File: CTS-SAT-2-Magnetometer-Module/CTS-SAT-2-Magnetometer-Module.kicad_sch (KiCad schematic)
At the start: 32 parts, among them J1 Conn_01x04_Pin, J2 SWD, SW1 SW_Push, U1 MMC5983MA, U2 LIS2MDL, U3 STM32F072C8Tx, U5 MIC5365-3.0YC5

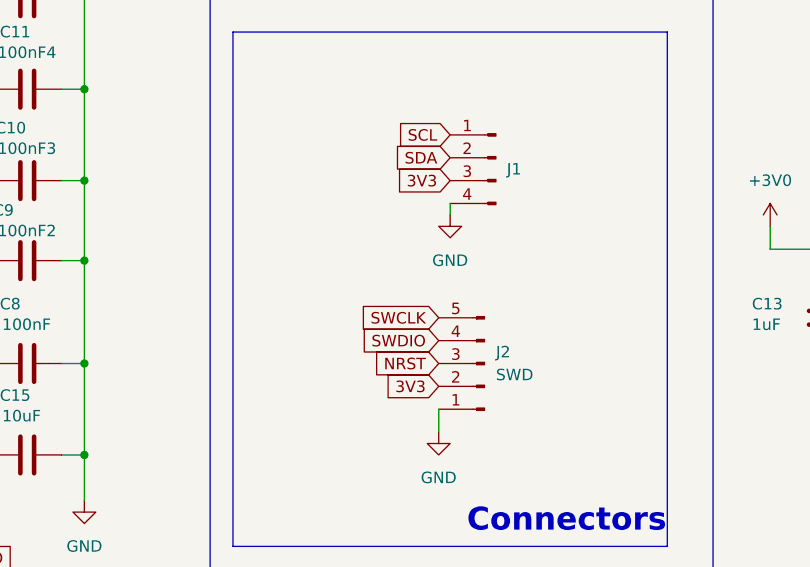
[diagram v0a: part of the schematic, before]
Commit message: FInished routing
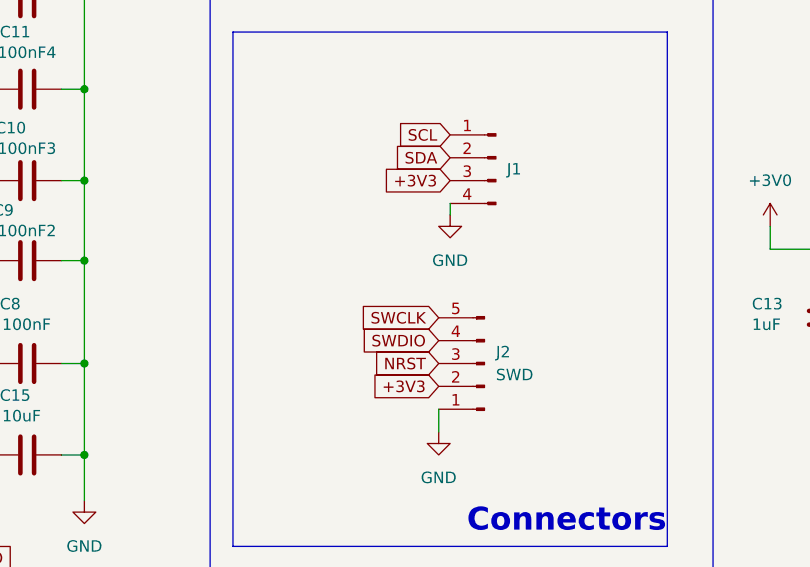
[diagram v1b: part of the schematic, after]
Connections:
- net +3V3: now also J1.3 (Pin_3), J2.2 (Pin_2)
- net 3V3: no longer J1.3 (Pin_3), J2.2 (Pin_2)
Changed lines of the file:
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@@
+		)
+	)
+	(global_label "+3V3"
+		(shape input)
+		(at 148.59 123.19 180)
+		(fields_autoplaced yes)
+		(effects
+			(font
+				(size 1.27 1.27)
+			)
+			(justify right)
+		)
+		(property "Intersheetrefs" "${INTERSHEET_REFS}"
+			(at 140.5248 123.19 0)
+			(hide yes)
+			(show_name no)
+			(do_not_autoplace no)
+			(effects
+				(font
+					(size 1.27 1.27)
+				)
+				(justify right)
+			)
+		)
+	)
+	(global_label "SWDIO"
+		(shape input)
+		(at 92.71 142.24 0)
+		(fields_autoplaced yes)
+		(effects
+			(font
+				(size 1.27 1.27)
+			)
+			(justify left)
+		)
+		(property "Intersheetrefs" "${INTERSHEET_REFS}"
+			(at 101.5614 142.24 0)
+			(hide yes)
+			(show_name no)
+			(do_not_autoplace no)
+			(effects
+				(font
+					(size 1.27 1.27)
+				)
+				(justify left)
+			)
+		)
+	)
+	(global_label "SWDIO"
+		(shape input)
+		(at 148.59 118.11 180)
+		(fields_autoplaced yes)
+		(effects
+			(font
+				(size 1.27 1.27)
+			)
+			(justify right)
+		)
+		(property "Intersheetrefs" "${INTERSHEET_REFS}"
+			(at 139.7386 118.11 0)
+			(hide yes)
+			(show_name no)
+			(do_not_autoplace no)
+			(effects
+				(font
+					(size 1.27 1.27)
+				)
+				(justify right)
+			)
+		)
+	)
+	(global_label "SCL"
+		(shape input)
+		(at 189.23 59.69 180)
+		(fields_autoplaced yes)
+		(effects
+			(font
+				(size 1.27 1.27)
+			)
+			(justify right)
+		)
+		(property "Intersheetrefs" "${INTERSHEET_REFS}"
+			(at 182.7372 59.69 0)
+			(hide yes)
+			(show_name no)
+			(do_not_autoplace no)
+			(effects
+				(font
+					(size 1.27 1.27)
+				)
+				(justify right)
+			)
+		)
+	)
+	(global_label "SWCLK"
+		(shape input)
+		(at 92.71 144.78 0)
+		(fields_autoplaced yes)
+		(effects
+			(font
+				(size 1.27 1.27)
+			)
+			(justify left)
+		)
+		(property "Intersheetrefs" "${INTERSHEET_REFS}"
+			(at 101.9242 144.78 0)
+			(hide yes)
+			(show_name no)
+			(do_not_autoplace no)
+			(effects
+				(font
+					(size 1.27 1.27)
+				)
+				(justify left)
+			)
+		)
+	)
+	(global_label "SDA"
+		(shape input)
+		(at 257.81 100.33 0)
+		(fields_autoplaced yes)
+		(effects
+			(font
+				(size 1.27 1.27)
+			)
+			(justify left)
+		)
+		(property "Intersheetrefs" "${INTERSHEET_REFS}"
+			(at 264.3633 100.33 0)
+			(hide yes)
+			(show_name no)
+			(do_not_autoplace no)
+			(effects
+				(font
+					(size 1.27 1.27)
+				)
+				(justify left)
+			)
+		)
+	)
+	(global_label "SDA"
+		(shape input)
+		(at 30.48 172.72 180)
+		(fields_autoplaced yes)
+		(effects
+			(font
+				(size 1.27 1.27)
+			)
+			(justify right)
+		)
+		(property "Intersheetrefs" "${INTERSHEET_REFS}"
+			(at 23.9267 172.72 0)
+			(hide yes)
+			(show_name no)
+			(do_not_autoplace no)
+			(effects
+				(font
+					(size 1.27 1.27)
+				)
+				(justify right)
+			)
 		)
 	)
 	(global_label "3V3"
 		(shape input)
-		(at 148.59 123.19 180)
-		(fields_autoplaced yes)
-		(effects
-			(font
-				(size 1.27 1.27)
-			)
-			(justify right)
-		)
-		(property "Intersheetrefs" "${INTERSHEET_REFS}"
-			(at 142.0972 123.19 0)
-			(hide yes)
-			(show_name no)
-			(do_not_autoplace no)
-			(effects
-				(font
-					(size 1.27 1.27)
-				)
-				(justify right)
-			)
-		)
-	)
-	(global_label "SWDIO"
-		(shape input)
-		(at 92.71 142.24 0)
-		(fields_autoplaced yes)
-		(effects
-			(font
-				(size 1.27 1.27)
-			)
-			(justify left)
-		)
-		(property "Intersheetrefs" "${INTERSHEET_REFS}"
-			(at 101.5614 142.24 0)
-			(hide yes)
-			(show_name no)
-			(do_not_autoplace no)
-			(effects
-				(font
-					(size 1.27 1.27)
-				)
-				(justify left)
-			)
-		)
-	)
-	(global_label "SWDIO"
-		(shape input)
-		(at 148.59 118.11 180)
-		(fields_autoplaced yes)
-		(effects
-			(font
-				(size 1.27 1.27)
-			)
-			(justify right)
-		)
-		(property "Intersheetrefs" "${INTERSHEET_REFS}"
-			(at 139.7386 118.11 0)
-			(hide yes)
-			(show_name no)
-			(do_not_autoplace no)
-			(effects
-				(font
-					(size 1.27 1.27)
-				)
-				(justify right)
-			)
-		)
-	)
-	(global_label "SCL"
-		(shape input)
-		(at 189.23 59.69 180)
-		(fields_autoplaced yes)
-		(effects
-			(font
-				(size 1.27 1.27)
-			)
-			(justify right)
-		)
-		(property "Intersheetrefs" "${INTERSHEET_REFS}"
-			(at 182.7372 59.69 0)
-			(hide yes)
-			(show_name no)
-			(do_not_autoplace no)
-			(effects
-				(font
-					(size 1.27 1.27)
-				)
-				(justify right)
-			)
-		)
-	)
-	(global_label "SWCLK"
-		(shape input)
-		(at 92.71 144.78 0)
-		(fields_autoplaced yes)
-		(effects
-			(font
-				(size 1.27 1.27)
-			)
-			(justify left)
-		)
-		(property "Intersheetrefs" "${INTERSHEET_REFS}"
-			(at 101.9242 144.78 0)
-			(hide yes)
-			(show_name no)
-			(do_not_autoplace no)
-			(effects
-				(font
-					(size 1.27 1.27)
-				)
-				(justify left)
-			)
-		)
-	)
-	(global_label "SDA"
-		(shape input)
-		(at 257.81 100.33 0)
-		(fields_autoplaced yes)
-		(effects
-			(font
-				(size 1.27 1.27)
-			)
-			(justify left)
-		)
-		(property "Intersheetrefs" "${INTERSHEET_REFS}"
-			(at 264.3633 100.33 0)
-			(hide yes)
-			(show_name no)
-			(do_not_autoplace no)
-			(effects
-				(font
-					(size 1.27 1.27)
-				)
-				(justify left)
-			)
-		)
-	)
-	(global_label "SDA"
-		(shape input)
-		(at 30.48 172.72 180)
-		(fields_autoplaced yes)
-		(effects
-			(font
-				(size 1.27 1.27)
-			)
-			(justify right)
-		)
-		(property "Intersheetrefs" "${INTERSHEET_REFS}"
-			(at 23.9267 172.72 0)
-			(hide yes)
-			(show_name no)
-			(do_not_autoplace no)
-			(effects
-				(font
-					(size 1.27 1.27)
-				)
-				(justify right)
-			)
-		)
-	)
-	(global_label "3V3"
-		(shape input)
 		(at 69.85 38.1 180)
 		(fields_autoplaced yes)
@@
 		)
 	)
-	(global_label "3V3"
+	(global_label "+3V3"
 		(shape input)
 		(at 149.86 100.33 180)
@@
 		)
 		(property "Intersheetrefs" "${INTERSHEET_REFS}"
-			(at 143.3672 100.33 0)
-			(hide yes)
-			(show_name no)
+			(at 141.7948 100.33 0)
+			(hide yes)
+			(show_name no)

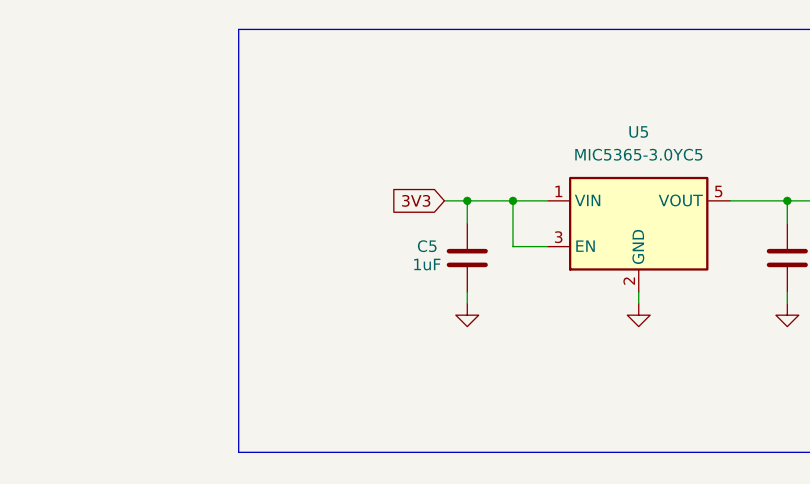
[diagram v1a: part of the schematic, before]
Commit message: Fixed a label
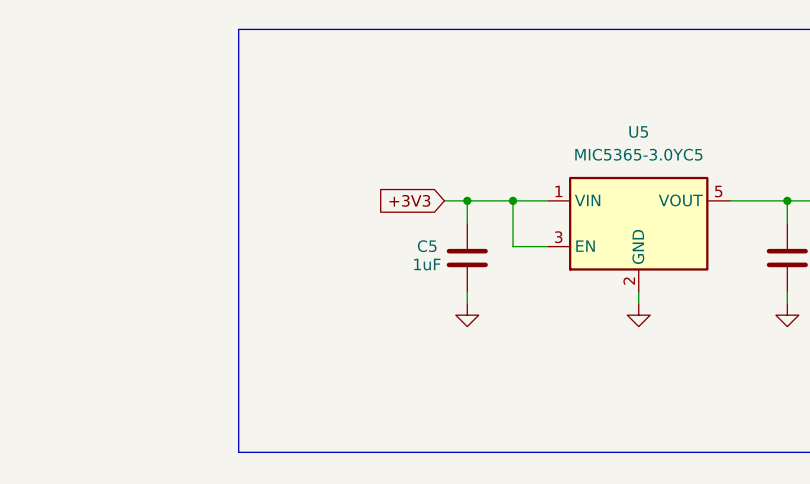
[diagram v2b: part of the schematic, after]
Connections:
- net 3V3 is gone; now on net +3V3: C5.1, U5.1 (VIN), U5.3 (EN)
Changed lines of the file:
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@@
 		)
 	)
-	(global_label "3V3"
+	(global_label "+3V3"
 		(shape input)
 		(at 69.85 38.1 180)
@@
 		)
 		(property "Intersheetrefs" "${INTERSHEET_REFS}"
-			(at 63.3572 38.1 0)
+			(at 61.7848 38.1 0)
 			(hide yes)
 			(show_name no)
